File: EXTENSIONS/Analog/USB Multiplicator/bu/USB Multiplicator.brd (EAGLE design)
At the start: 58 x 71 mm, 10 parts, among them X1 USB-A

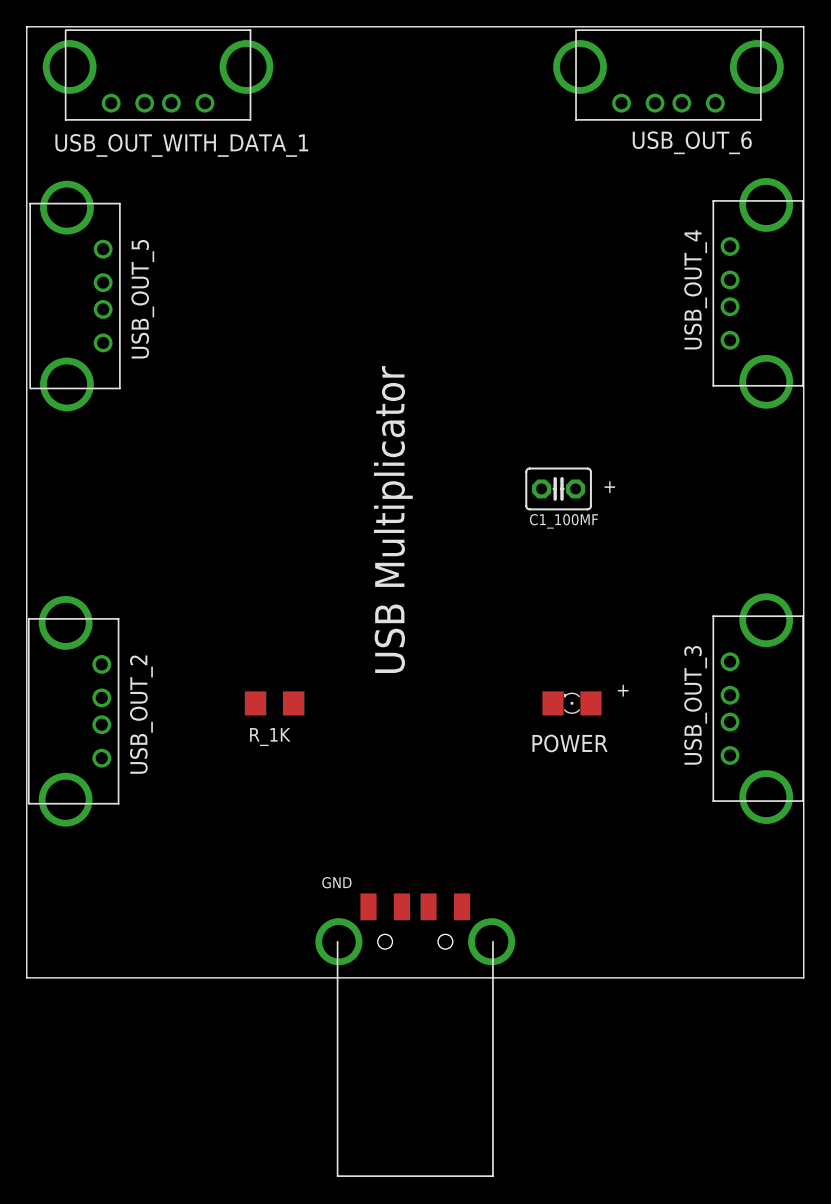
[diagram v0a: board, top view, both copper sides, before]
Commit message: Create USB multiplicator v2 big
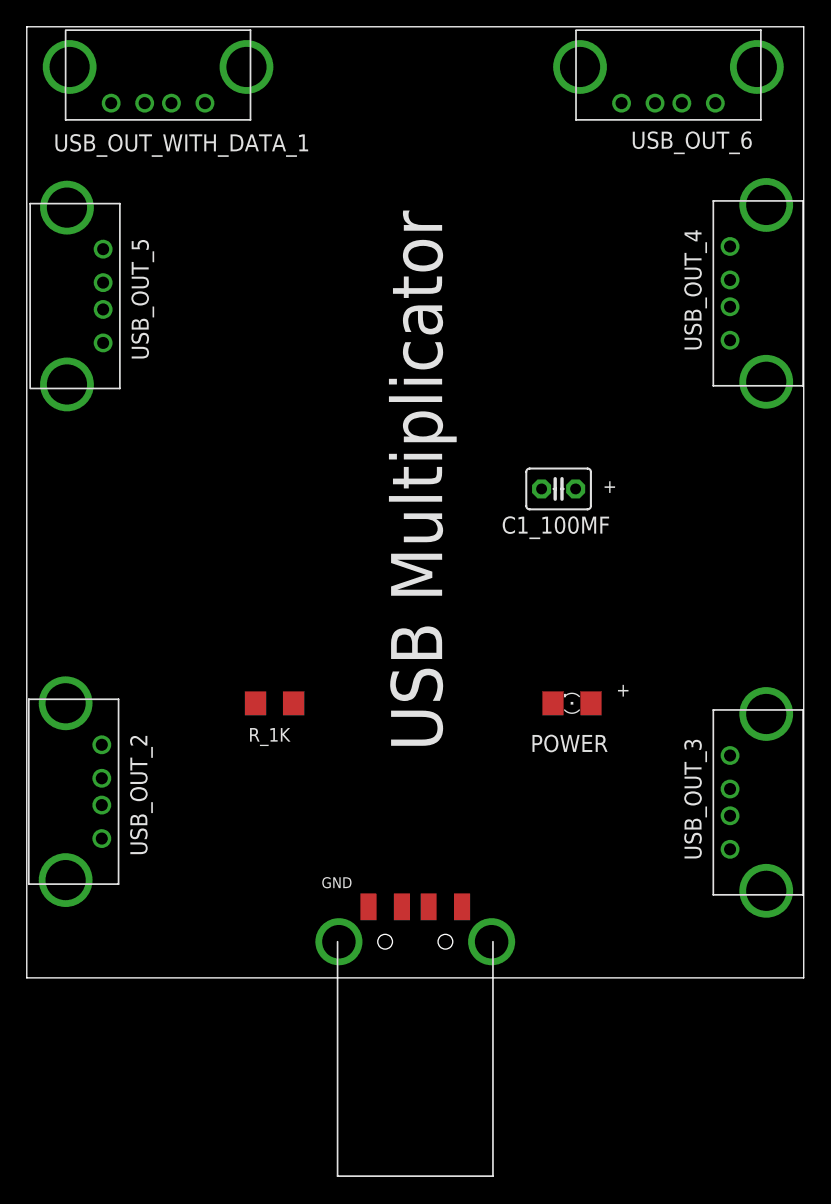
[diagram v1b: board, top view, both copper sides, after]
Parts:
- moved USB_OUT_3 7.00 mm to (53.2, 32.0)
- moved USB_OUT_2 6.00 mm to (8.90, 19.0)
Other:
- board text added: "PCBv3 - 2019.12"
- board text removed: "PCBv2 - 2019.08"
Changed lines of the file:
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@@
 <wire x1="60" y1="83" x2="2" y2="83" width="0" layer="20"/>
 <wire x1="2" y1="83" x2="2" y2="12" width="0" layer="20"/>
-<text x="17" y="50.2" size="1.778" layer="26" rot="SMR90" align="center">USB Multiplicator
+<text x="31" y="55.2" size="3.81" layer="26" rot="SMR90" align="center">USB Multiplicator
 MadeInTheUSB.net </text>
-<text x="22.5" y="18" size="1.27" layer="26" rot="MR90">PCBv2 - 2019.08</text>
+<text x="30.5" y="23" size="1.27" layer="26" rot="MR0" align="center">PCBv3 - 2019.12</text>
 <text x="24" y="18.7" size="0.8128" layer="25">GND</text>
 <text x="45" y="48.2" size="1.016" layer="25">+</text>
 <text x="46" y="33" size="1.016" layer="25">+</text>
 <text x="42.5" y="29.5" size="1.27" layer="25" align="center">POWER</text>
-<text x="29.1" y="46.1" size="2.1844" layer="25" rot="R90" align="center">USB Multiplicator</text>
+<text x="31.1" y="49.1" size="3.81" layer="25" rot="R90" align="center">USB Multiplicator</text>
 </plain>
 <attributes>
@@
 </element>
 <element name="C1_100MF" library="adafruit" package="C025-030X050" value="" x="41.7" y="48.5" smashed="yes">
-<attribute name="NAME" x="39.5" y="45.8" size="0.8128" layer="25" ratio="10"/>
+<attribute name="NAME" x="41.5" y="45.8" size="1.27" layer="25" ratio="10" align="center"/>
 <attribute name="VALUE" x="39.414" y="45.452" size="1.27" layer="27" ratio="10"/>
 </element>
@@
 <attribute name="NAME" x="4" y="73.7" size="1.27" layer="25"/>
 </element>
-<element name="USB_OUT_2" library="STUNTAZ" package="USB-FEMALE-A-PTH" value="USB" x="8.9" y="25" smashed="yes" rot="R90">
-<attribute name="NAME" x="11" y="27.1" size="1.27" layer="25" rot="R90"/>
-</element>
-<element name="USB_OUT_3" library="STUNTAZ" package="USB-FEMALE-A-PTH" value="USB" x="53.2" y="39" smashed="yes" rot="R270">
-<attribute name="NAME" x="51.1" y="36.9" size="1.27" layer="25" rot="R270"/>
+<element name="USB_OUT_2" library="STUNTAZ" package="USB-FEMALE-A-PTH" value="USB" x="8.9" y="19" smashed="yes" rot="R90">
+<attribute name="NAME" x="11" y="21.1" size="1.27" layer="25" rot="R90"/>
+</element>
+<element name="USB_OUT_3" library="STUNTAZ" package="USB-FEMALE-A-PTH" value="USB" x="53.2" y="32" smashed="yes" rot="R270">
+<attribute name="NAME" x="51.1" y="29.9" size="1.27" layer="25" rot="R270"/>
 </element>
 <element name="USB_OUT_4" library="STUNTAZ" package="USB-FEMALE-A-PTH" value="USB" x="53.2" y="70" smashed="yes" rot="R270">
@@
 <contactref element="USB_OUT_6" pad="GND"/>
 <wire x1="54.5" y1="66.6" x2="46.4" y2="77.3" width="0" layer="19" extent="1-1"/>
-<wire x1="54.5" y1="35.6" x2="54.5" y2="66.6" width="0" layer="19" extent="1-1"/>
-<wire x1="27.5" y1="17.3" x2="54.5" y2="35.6" width="0" layer="19" extent="1-1"/>
-<wire x1="40.43" y1="48.5" x2="27.5" y2="17.3" width="0" layer="19" extent="1-1"/>
-<wire x1="7.6" y1="28.4" x2="40.43" y2="48.5" width="0" layer="19" extent="1-1"/>
-<wire x1="19.078" y1="32.5" x2="7.6" y2="28.4" width="0" layer="19" extent="1-1"/>
-<wire x1="7.7" y1="59.4" x2="7.6" y2="28.4" width="0" layer="19" extent="1-1"/>
+<wire x1="40.43" y1="48.5" x2="54.5" y2="66.6" width="0" layer="19" extent="1-1"/>
+<wire x1="54.5" y1="28.6" x2="40.43" y2="48.5" width="0" layer="19" extent="1-1"/>
+<wire x1="19.078" y1="32.5" x2="40.43" y2="48.5" width="0" layer="19" extent="1-1"/>
+<wire x1="7.6" y1="22.4" x2="19.078" y2="32.5" width="0" layer="19" extent="1-1"/>
+<wire x1="27.5" y1="17.3" x2="19.078" y2="32.5" width="0" layer="19" extent="1-1"/>
+<wire x1="7.7" y1="59.4" x2="19.078" y2="32.5" width="0" layer="19" extent="1-1"/>
 <wire x1="8.3" y1="77.3" x2="7.7" y2="59.4" width="0" layer="19" extent="1-1"/>
 </signal>
@@
 <contactref element="USB_OUT_6" pad="VBUS"/>
 <wire x1="54.5" y1="59.6" x2="53.4" y2="77.3" width="0" layer="19" extent="1-1"/>
-<wire x1="54.5" y1="28.6" x2="54.5" y2="59.6" width="0" layer="19" extent="1-1"/>
-<wire x1="34.5" y1="17.3" x2="54.5" y2="28.6" width="0" layer="19" extent="1-1"/>
-<wire x1="44.122" y1="32.5" x2="34.5" y2="17.3" width="0" layer="19" extent="1-1"/>
-<wire x1="42.97" y1="48.5" x2="44.122" y2="32.5" width="0" layer="19" extent="1-1"/>
-<wire x1="7.6" y1="35.4" x2="42.97" y2="48.5" width="0" layer="19" extent="1-1"/>
-<wire x1="7.7" y1="66.4" x2="7.6" y2="35.4" width="0" layer="19" extent="1-1"/>
+<wire x1="42.97" y1="48.5" x2="54.5" y2="59.6" width="0" layer="19" extent="1-1"/>
+<wire x1="44.122" y1="32.5" x2="42.97" y2="48.5" width="0" layer="19" extent="1-1"/>
+<wire x1="54.5" y1="21.6" x2="44.122" y2="32.5" width="0" layer="19" extent="1-1"/>
+<wire x1="34.5" y1="17.3" x2="44.122" y2="32.5" width="0" layer="19" extent="1-1"/>
+<wire x1="7.6" y1="29.4" x2="34.5" y2="17.3" width="0" layer="19" extent="1-1"/>
+<wire x1="7.7" y1="66.4" x2="7.6" y2="29.4" width="0" layer="19" extent="1-1"/>
 <wire x1="15.3" y1="77.3" x2="7.7" y2="66.4" width="0" layer="19" extent="1-1"/>
 </signal>
